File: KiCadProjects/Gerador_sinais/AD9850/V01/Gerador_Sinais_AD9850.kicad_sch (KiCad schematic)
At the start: 41 parts, among them J1 alimentacao analogica, J10 teclado matricial, J11 botoes_selecao, J2 sinais analogicos, J3 comunicacao / sinais digitais, J4 3.3V STM32, J5 5.0V STM32, J6 Select SinA, J7 Select SinB, J8 Squad_wave, J9 Encoder KY-040, U1 AD9850_module, U2 BluePill_STM32F103C, U3 AD828AN, U4 X9c10x, U5 X9c10x, U6 AD828AN

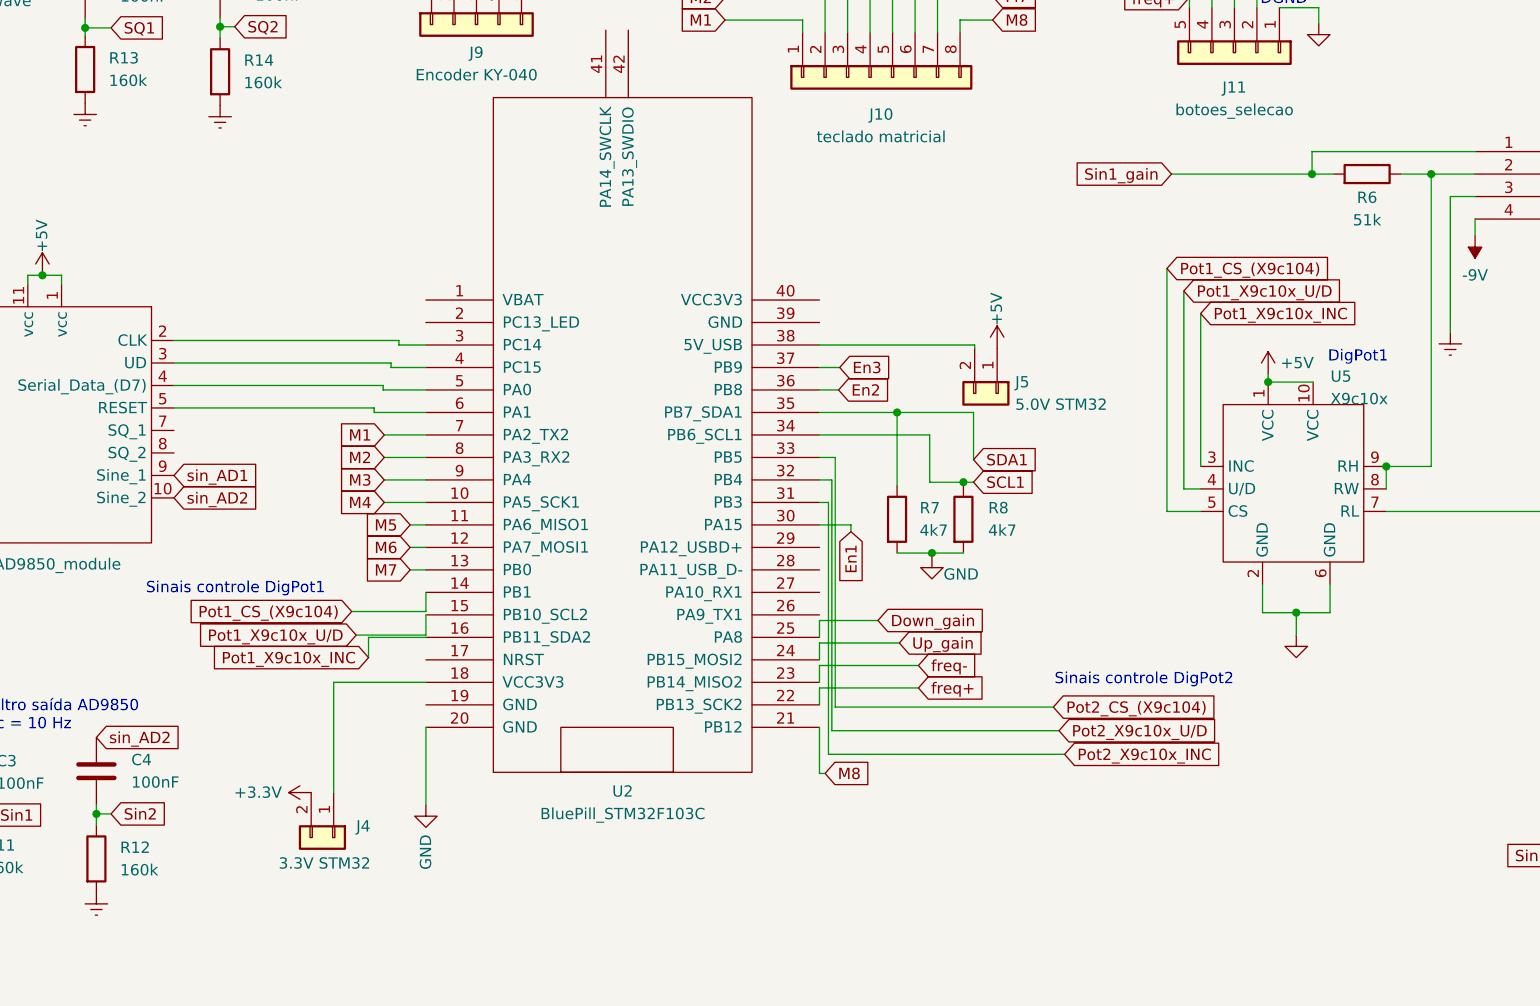
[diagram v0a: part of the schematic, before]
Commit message: todas conexoes feitas
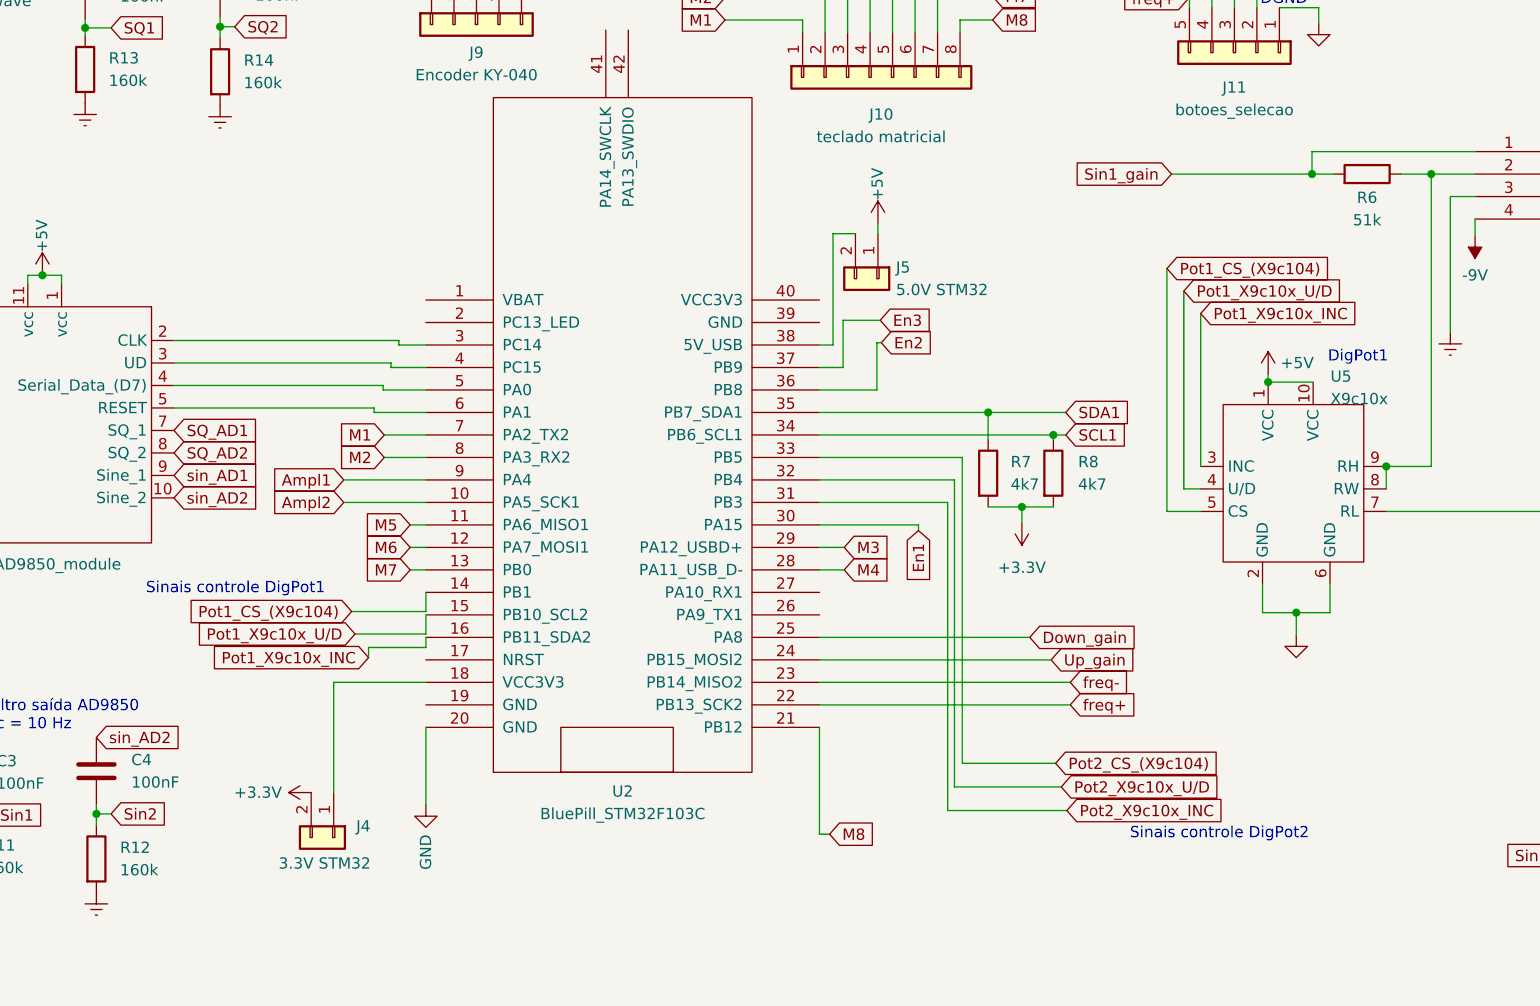
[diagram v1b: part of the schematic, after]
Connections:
- net +3.3V: now also R7.2, R8.2
- net Ampl1: now also U2.9 (PA4)
- net Ampl2: now also U2.10 (PA5_SCK1)
- net Earth: no longer R7.2, R8.2
- net M3: now also U2.29 (PA12_USBD+); no longer U2.9 (PA4)
- net M4: now also U2.28 (PA11_USB_D-); no longer U2.10 (PA5_SCK1)
- net SQ_AD1: now also U1.7 (SQ_1)
- net SQ_AD2: now also U1.8 (SQ_2)
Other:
- moved on the sheet: J5, R7, R8
